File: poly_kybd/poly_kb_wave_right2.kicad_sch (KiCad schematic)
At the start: 47 parts, among them J37 FH34SRJ-12S-0.5SH, J38 Conn_01x05, J39 FH12-30S-0.5SH, SW1 RotaryEncoder_Switch, U2 TD6811, U3 MT9700

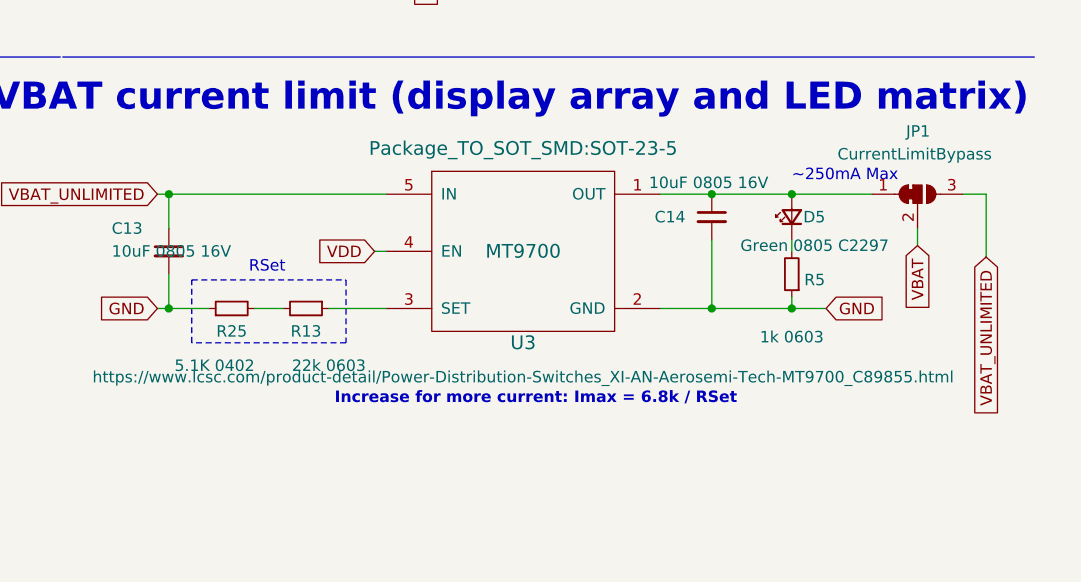
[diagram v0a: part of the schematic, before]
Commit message: Added latest gerber files, latest STLs and updated readme
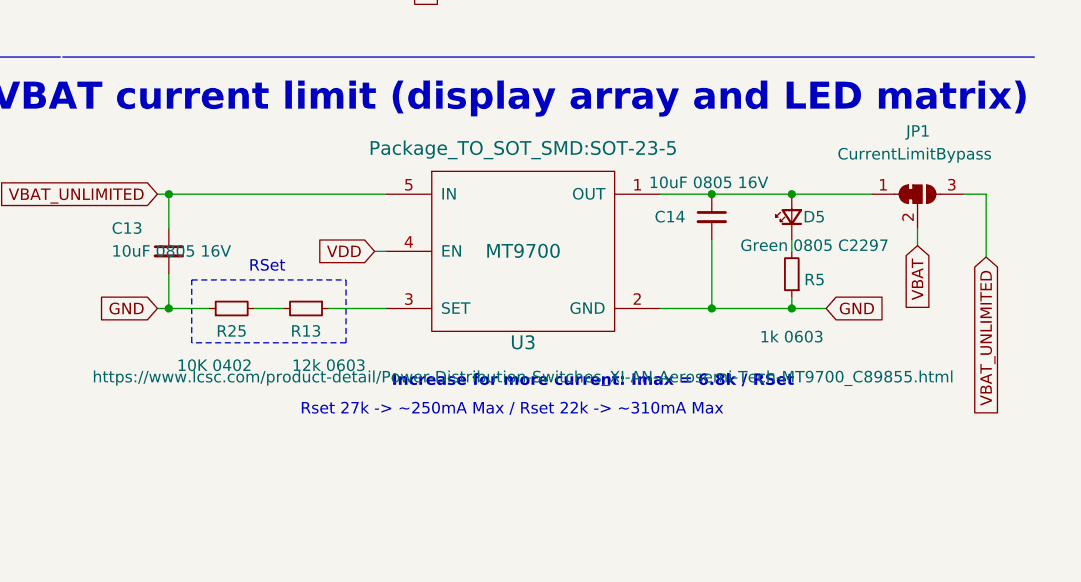
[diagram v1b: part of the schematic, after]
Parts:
- R13: value 22k 0603 -> 12k 0603; JLC (none) -> C22790; MPN C31850 -> C22790
- R25: value 5.1K 0402 -> 10K 0402; MPN C25905 -> C25744
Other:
- note added: "Rset 27k -> ~250mA Max / Rset 22k -> ~310mA Max"
- note removed: "~250mA Max"
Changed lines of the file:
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@@
     (effects (font (size 3 3) (thickness 0.6) bold) (justify left bottom))
   )
-  (text "Increase for more current: Imax = 6.8k / RSet" (at 504.19 374.015 0)
+  (text "Increase for more current: Imax = 6.8k / RSet" (at 510.54 372.11 0)
     (effects (font (size 1.27 1.27) bold) (justify left bottom))
   )
@@
     (effects (font (size 3 3) (thickness 0.6) bold) (justify left bottom))
   )
-  (text "~250mA Max" (at 554.99 349.25 0)
+  (text "Rset 27k -> ~250mA Max / Rset 22k -> ~310mA Max" (at 500.38 375.285 0)
     (effects (font (size 1.27 1.27)) (justify left bottom))
   )
@@
       (effects (font (size 1.27 1.27)))
     )
-    (property "Value" "5.1K 0402" (at 490.855 369.57 90)
+    (property "Value" "10K 0402" (at 490.855 369.57 90)
       (effects (font (size 1.27 1.27)))
     )
@@
       (effects (font (size 1.27 1.27)) hide)
     )
-    (property "MPN" "C25905" (at 492.76 363.22 0)
+    (property "MPN" "C25744" (at 492.76 363.22 0)
       (effects (font (size 1.27 1.27)) hide)
     )
@@
       (effects (font (size 1.27 1.27)))
     )
-    (property "Value" "22k 0603" (at 503.555 369.57 90)
+    (property "Value" "12k 0603" (at 503.555 369.57 90)
       (effects (font (size 1.27 1.27)))
     )
@@
       (effects (font (size 1.27 1.27)) hide)
     )
-    (property "MPN" "C31850" (at 501.015 363.22 0)
+    (property "MPN" "C22790" (at 501.015 363.22 0)
       (effects (font (size 1.27 1.27)) hide)
     )
-    (property "JLC" "" (at 501.015 363.22 0)
+    (property "JLC" "C22790" (at 501.015 363.22 0)
       (effects (font (size 1.27 1.27)) hide)
     )
